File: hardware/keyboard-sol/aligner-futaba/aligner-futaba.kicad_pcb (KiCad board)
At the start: 2 copper layers, 428.6 x 117.7 mm, 96 parts, among them SW10 TAB: 1.25x, SW11 I, SW12 2, SW13 Zero, SW14 Q, SW15 O, SW16 3, SW17 Dash, SW18 W, SW19 P, SW20 4, SW21 Caret, SW22 E, SW23 AT, SW24 5, SW25 LT Bracket, SW26 R, SW27 Return: 1.5x, SW28 6, SW29 Backslash, SW30 T, SW31 Line Feed, SW32 7, SW33 RT Bracket, SW34 Y, SW35 Load, SW36 LT Ctrl, SW37 J, SW38 Upper Case: 1.5x, SW39 M, SW4 ESC: 1.75x, SW40 Shift Lock: 1.5x, SW41 K, SW42 LT Shift: 1.5x, SW43 Comma, SW44 A, SW45 L, SW46 Z, SW47 Period, SW48 S, SW49 Semicolon, SW5 8, SW50 X, SW51 Slash, SW52 D, SW53 Colon, SW54 C, SW55 RT Shift: 2x, SW56 F, SW57 DEL, SW58 V, SW59 Mode Select: 1.75x, SW6 BREAK, SW60 G, SW61 Repeat: 1.25x, SW62 B, SW63 H, SW64 RT Ctrl, SW65 N, SW66 Local, SW67 NP Dash, SW68 NP 4, SW69 NP Zero, SW7 U, SW70 Up Arrow, SW71 NP 7, SW72 NP 1, SW73 NP period, SW74 LT Arrow, SW75 NP asterisk, SW76 NP 5, SW77 NP plus, SW78 Spacebar, SW79 NP 8, SW8 1, SW80 NP 2, SW81 RT Arrow, SW82 NP divide, SW83 NP 6, SW84 Down Arrow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

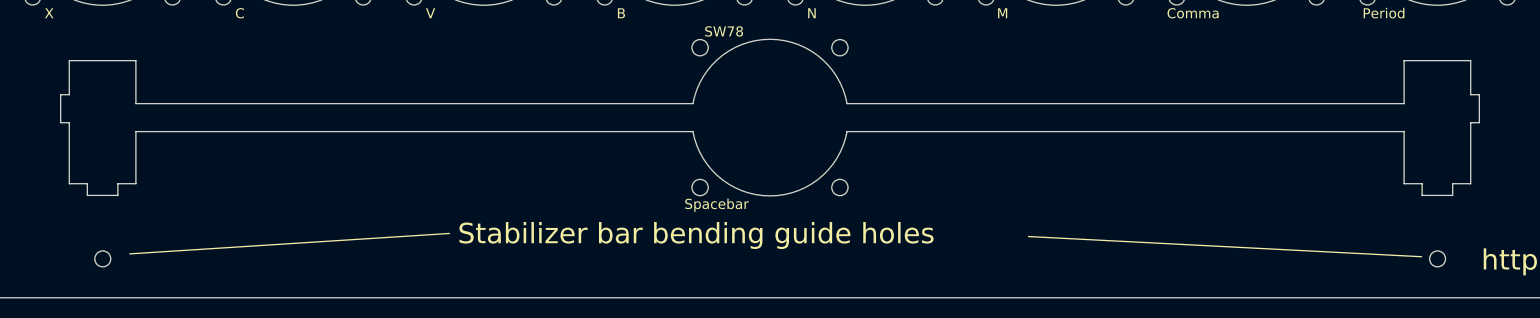
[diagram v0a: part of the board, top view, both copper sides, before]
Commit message: Hole size adjustment
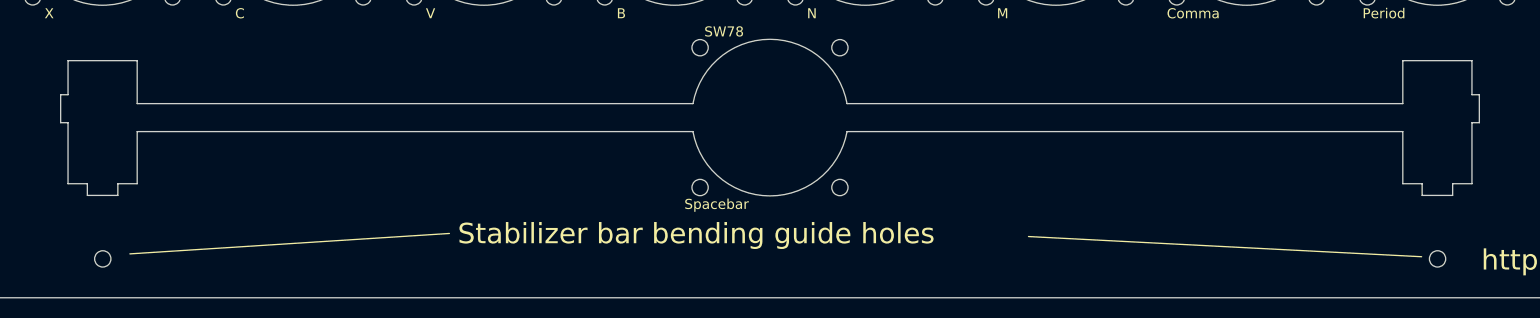
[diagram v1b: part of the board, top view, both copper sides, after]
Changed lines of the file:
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@@
     (mod_text_size 1 1)
     (mod_text_width 0.15)
-    (pad_size 1.5875 1.5875)
-    (pad_drill 1.5875)
+    (pad_size 1.6256 1.6256)
+    (pad_drill 1.6256)
     (pad_to_mask_clearance 0)
     (aux_axis_origin 61.4172 179.1081)
@@
       (effects (font (size 1 1) (thickness 0.15)))
     )
-    (fp_line (start -63.3476 -5.6896) (end -63.3476 -1.397) (layer Edge.Cuts) (width 0.12))
-    (fp_line (start -70.0024 -5.6896) (end -63.3476 -5.6896) (layer Edge.Cuts) (width 0.12))
-    (fp_line (start -70.0024 -2.286) (end -70.0024 -5.6896) (layer Edge.Cuts) (width 0.12))
-    (fp_line (start -70.866 -2.286) (end -70.0024 -2.286) (layer Edge.Cuts) (width 0.12))
-    (fp_line (start -70.866 0.508) (end -70.866 -2.286) (layer Edge.Cuts) (width 0.12))
-    (fp_line (start -70.0024 0.508) (end -70.866 0.508) (layer Edge.Cuts) (width 0.12))
-    (fp_line (start -70.0024 6.604) (end -70.0024 0.508) (layer Edge.Cuts) (width 0.12))
-    (fp_line (start -68.199 6.604) (end -70.0024 6.604) (layer Edge.Cuts) (width 0.12))
-    (fp_line (start -68.199 7.7724) (end -68.199 6.604) (layer Edge.Cuts) (width 0.12))
-    (fp_line (start -65.151 7.7724) (end -68.199 7.7724) (layer Edge.Cuts) (width 0.12))
-    (fp_line (start -65.151 6.604) (end -65.151 7.7724) (layer Edge.Cuts) (width 0.12))
-    (fp_line (start -63.3476 6.604) (end -65.151 6.604) (layer Edge.Cuts) (width 0.12))
-    (fp_line (start -63.3476 1.397) (end -63.3476 6.604) (layer Edge.Cuts) (width 0.12))
-    (fp_line (start 63.3476 6.604) (end 63.3476 1.397) (layer Edge.Cuts) (width 0.12))
-    (fp_line (start 65.151 6.604) (end 63.3476 6.604) (layer Edge.Cuts) (width 0.12))
-    (fp_line (start 65.151 7.7724) (end 65.151 6.604) (layer Edge.Cuts) (width 0.12))
-    (fp_line (start 68.199 7.7724) (end 65.151 7.7724) (layer Edge.Cuts) (width 0.12))
-    (fp_line (start 68.199 6.604) (end 68.199 7.7724) (layer Edge.Cuts) (width 0.12))
-    (fp_line (start 70.0024 6.604) (end 68.199 6.604) (layer Edge.Cuts) (width 0.12))
-    (fp_line (start 70.0024 0.508) (end 70.0024 6.604) (layer Edge.Cuts) (width 0.12))
-    (fp_line (start 70.866 0.508) (end 70.0024 0.508) (layer Edge.Cuts) (width 0.12))
-    (fp_line (start 70.866 -2.286) (end 70.866 0.508) (layer Edge.Cuts) (width 0.12))
-    (fp_line (start 70.0024 -2.286) (end 70.866 -2.286) (layer Edge.Cuts) (width 0.12))
-    (fp_line (start 70.0024 -5.6896) (end 70.0024 -2.286) (layer Edge.Cuts) (width 0.12))
-    (fp_line (start 63.3476 -5.6896) (end 70.0024 -5.6896) (layer Edge.Cuts) (width 0.12))
-    (fp_line (start 63.3476 -1.397) (end 63.3476 -5.6896) (layer Edge.Cuts) (width 0.12))
-    (fp_line (start 7.697216 1.397) (end 63.3476 1.397) (layer Edge.Cuts) (width 0.12))
-    (fp_line (start 7.697216 -1.397) (end 63.3476 -1.397) (layer Edge.Cuts) (width 0.12))
-    (fp_line (start -63.3476 -1.397) (end -7.697216 -1.397) (layer Edge.Cuts) (width 0.12))
-    (fp_line (start -63.3476 1.397) (end -7.697216 1.397) (layer Edge.Cuts) (width 0.12))
     (fp_text user MX_space_aligner (at -0.6096 7.9248) (layer B.Fab)
       (effects (font (size 1 1) (thickness 0.15)))
@@
     (fp_arc (start 0 0) (end 7.697216 -1.397) (angle -159.4) (layer Edge.Cuts) (width 0.12))
     (fp_arc (start 0 0) (end -7.697216 1.397) (angle -159.4) (layer Edge.Cuts) (width 0.12))
+    (fp_line (start -63.2206 -5.6896) (end -63.2206 -1.397) (layer Edge.Cuts) (width 0.12))
+    (fp_line (start -70.1294 -5.6896) (end -63.2206 -5.6896) (layer Edge.Cuts) (width 0.12))
+    (fp_line (start -70.1294 -2.286) (end -70.1294 -5.6896) (layer Edge.Cuts) (width 0.12))
+    (fp_line (start -70.866 -2.286) (end -70.1294 -2.286) (layer Edge.Cuts) (width 0.12))
+    (fp_line (start -70.866 0.508) (end -70.866 -2.286) (layer Edge.Cuts) (width 0.12))
+    (fp_line (start -70.1294 0.508) (end -70.866 0.508) (layer Edge.Cuts) (width 0.12))
+    (fp_line (start -70.1294 6.604) (end -70.1294 0.508) (layer Edge.Cuts) (width 0.12))
+    (fp_line (start -68.199 6.604) (end -70.1294 6.604) (layer Edge.Cuts) (width 0.12))
+    (fp_line (start -68.199 7.7724) (end -68.199 6.604) (layer Edge.Cuts) (width 0.12))
+    (fp_line (start -65.151 7.7724) (end -68.199 7.7724) (layer Edge.Cuts) (width 0.12))
+    (fp_line (start -65.151 6.604) (end -65.151 7.7724) (layer Edge.Cuts) (width 0.12))
+    (fp_line (start -63.2206 6.604) (end -65.151 6.604) (layer Edge.Cuts) (width 0.12))
+    (fp_line (start -63.2206 1.397) (end -63.2206 6.604) (layer Edge.Cuts) (width 0.12))
+    (fp_line (start 63.2206 6.604) (end 63.2206 1.397) (layer Edge.Cuts) (width 0.12))
+    (fp_line (start 65.151 6.604) (end 63.2206 6.604) (layer Edge.Cuts) (width 0.12))
+    (fp_line (start 65.151 7.7724) (end 65.151 6.604) (layer Edge.Cuts) (width 0.12))
+    (fp_line (start 68.199 7.7724) (end 65.151 7.7724) (layer Edge.Cuts) (width 0.12))
+    (fp_line (start 68.199 6.604) (end 68.199 7.7724) (layer Edge.Cuts) (width 0.12))
+    (fp_line (start 70.1294 6.604) (end 68.199 6.604) (layer Edge.Cuts) (width 0.12))
+    (fp_line (start 70.1294 0.508) (end 70.1294 6.604) (layer Edge.Cuts) (width 0.12))
+    (fp_line (start 70.866 0.508) (end 70.1294 0.508) (layer Edge.Cuts) (width 0.12))
+    (fp_line (start 70.866 -2.286) (end 70.866 0.508) (layer Edge.Cuts) (width 0.12))
+    (fp_line (start 70.1294 -2.286) (end 70.866 -2.286) (layer Edge.Cuts) (width 0.12))
+    (fp_line (start 70.1294 -5.6896) (end 70.1294 -2.286) (layer Edge.Cuts) (width 0.12))
+    (fp_line (start 63.2206 -5.6896) (end 70.1294 -5.6896) (layer Edge.Cuts) (width 0.12))
+    (fp_line (start 63.2206 -1.397) (end 63.2206 -5.6896) (layer Edge.Cuts) (width 0.12))
+    (fp_line (start 7.697216 1.397) (end 63.2206 1.397) (layer Edge.Cuts) (width 0.12))
+    (fp_line (start 7.697216 -1.397) (end 63.2206 -1.397) (layer Edge.Cuts) (width 0.12))
+    (fp_line (start -63.2206 -1.397) (end -7.697216 -1.397) (layer Edge.Cuts) (width 0.12))
+    (fp_line (start -63.2206 1.397) (end -7.697216 1.397) (layer Edge.Cuts) (width 0.12))
     (pad "" np_thru_hole circle (at -6.985 6.985) (size 1.6256 1.6256) (drill 1.6256) (layers *.Cu *.Mask))
     (pad "" np_thru_hole circle (at -6.985 -6.985) (size 1.6256 1.6256) (drill 1.6256) (layers *.Cu *.Mask))
@@
       (effects (font (size 1 1) (thickness 0.15)))
     )
-    (pad "" np_thru_hole circle (at 0 0) (size 1.5875 1.5875) (drill 1.5875) (layers *.Cu *.Mask))
+    (pad "" np_thru_hole circle (at 0 0) (size 1.6256 1.6256) (drill 1.6256) (layers *.Cu *.Mask))
   )
   (module MountingHole:MountingHole_3.2mm_M3 (layer F.Cu)
@@
       (effects (font (size 1 1) (thickness 0.15)))
     )
-    (pad "" np_thru_hole circle (at 0 0) (size 1.5875 1.5875) (drill 1.5875) (layers *.Cu *.Mask))
+    (pad "" np_thru_hole circle (at 0 0) (size 1.6256 1.6256) (drill 1.6256) (layers *.Cu *.Mask))
   )
   (module unikbd:Futaba_2u_Cherry_aligner locked (layer F.Cu)
